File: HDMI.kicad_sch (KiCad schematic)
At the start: 103 parts, among them J3 Conn_01x03_Pin, J32 HDMI_D_1.4, J4 Conn_02x01, Q11 2N7002, Q12 2SK3018, Q13 2SK3018, Q14 2SK3018, U1 ADV7623BSTZ, U2 NC7SZ125M5, U43 TPAZ1023-04F, U44 TPAZ1023-04F, Y3 ABM8G-28.63636MHZ-18-D2Y-T

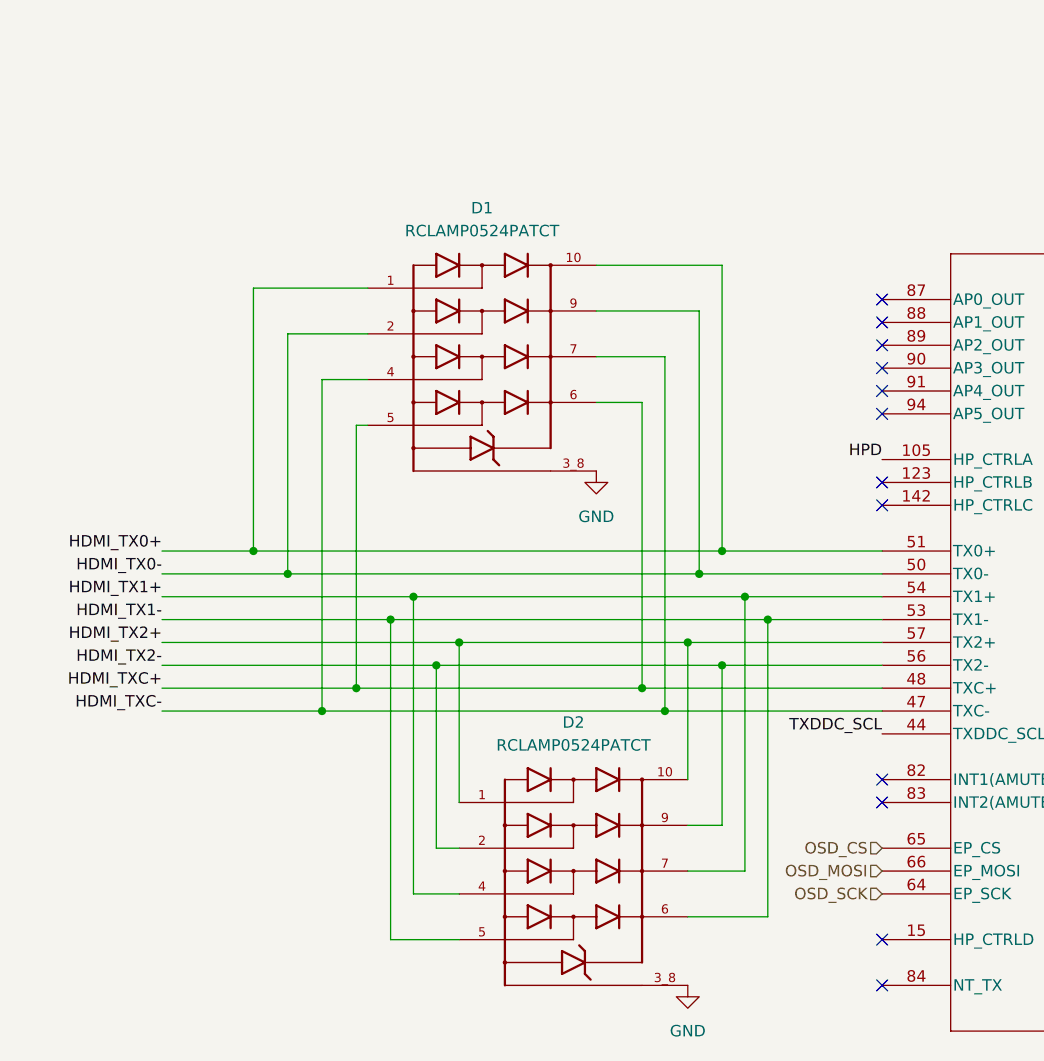
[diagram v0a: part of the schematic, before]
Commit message: some power stuff (unfinished)
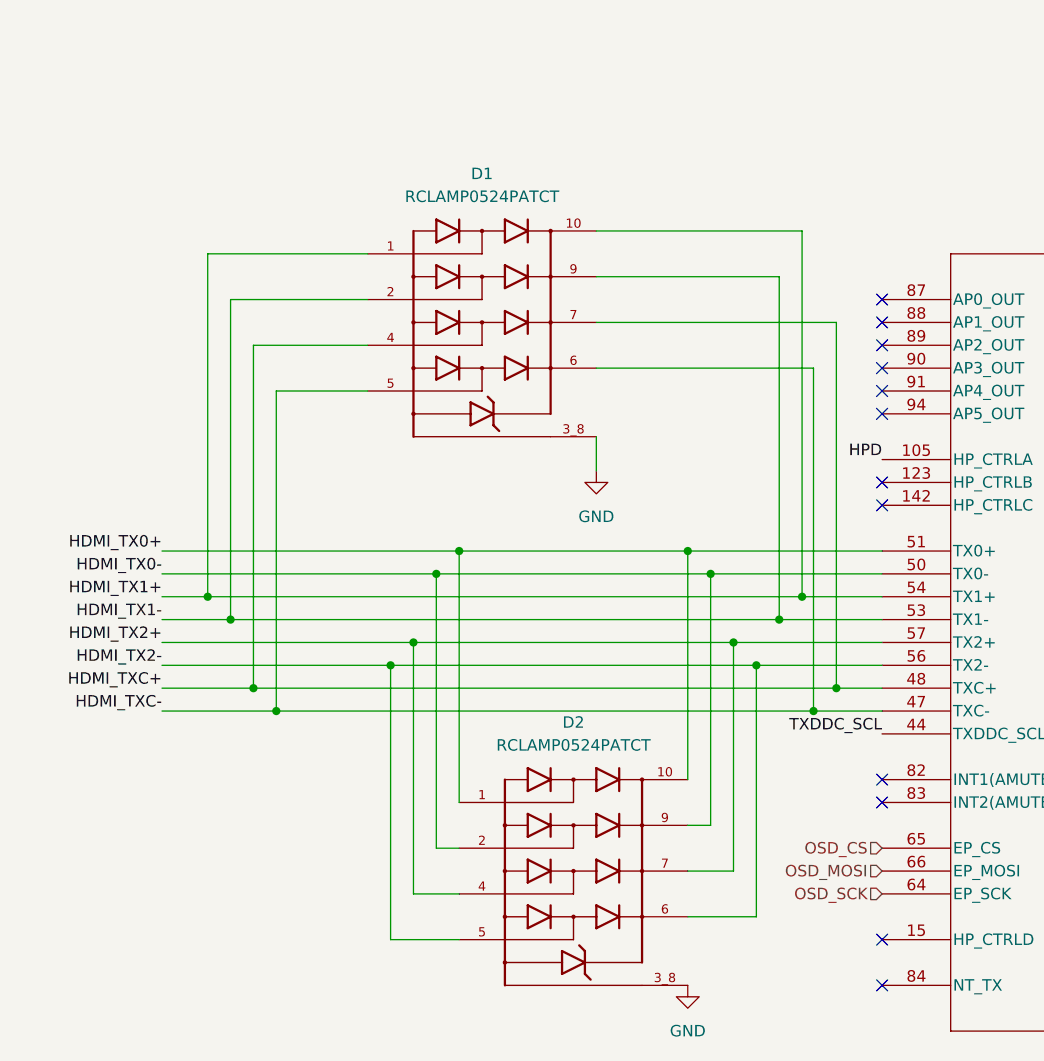
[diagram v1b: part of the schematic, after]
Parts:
- D1: footprint RCLAMP0524PATCT:DIO_RCLAMP0524PATCT -> HDMI:DIO_RCLAMP0524PATCT
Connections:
- net HDMI_TX0+: now also D2.1, D2.10; no longer D1.1, D1.10
- net HDMI_TX0-: now also D2.2, D2.9; no longer D1.2, D1.9
- net HDMI_TX1+: now also D1.1, D1.10; no longer D2.4, D2.7
- net HDMI_TX1-: now also D1.2, D1.9; no longer D2.5, D2.6
- net HDMI_TX2+: now also D2.4, D2.7; no longer D2.1, D2.10
- net HDMI_TX2-: now also D2.5, D2.6; no longer D2.2, D2.9
- net HDMI_TXC+: now also D1.4, D1.7; no longer D1.5, D1.6
- net HDMI_TXC-: now also D1.5, D1.6; no longer D1.4, D1.7
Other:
- moved on the sheet: D1
